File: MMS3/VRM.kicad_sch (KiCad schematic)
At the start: 32 parts, among them U3 TPS54560BDDA

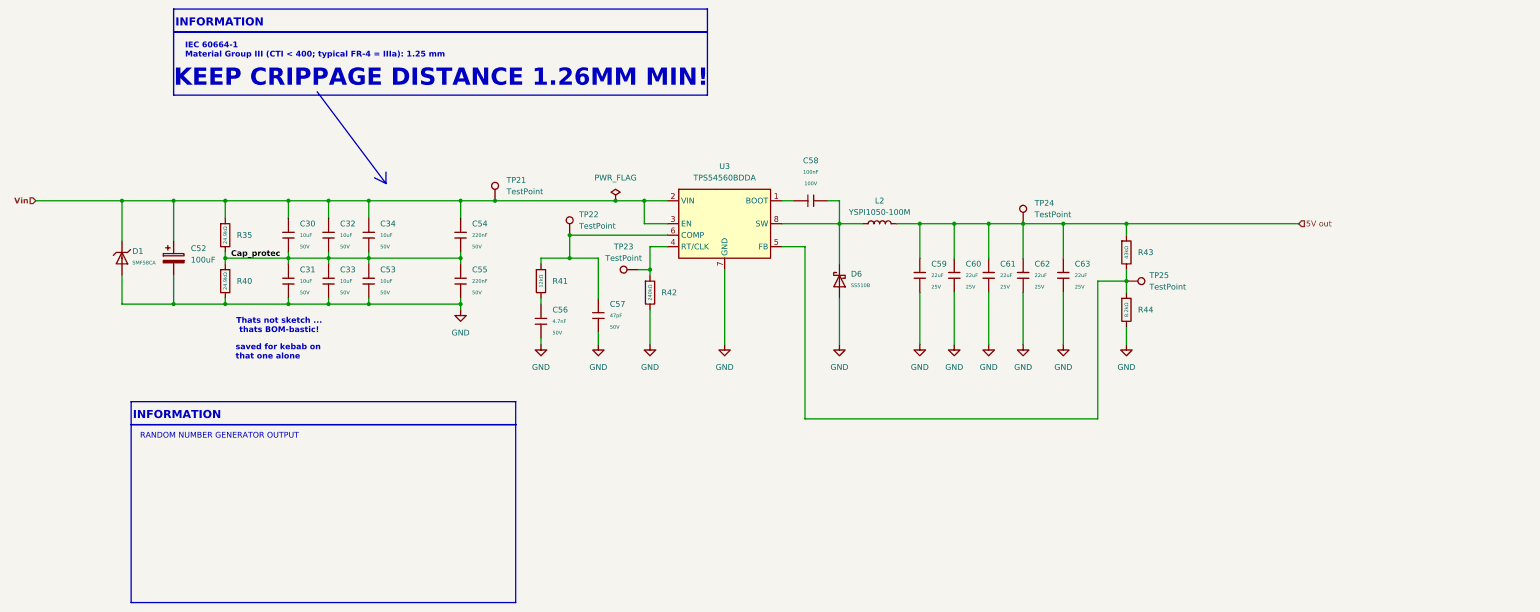
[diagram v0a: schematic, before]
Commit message: initial PCB update
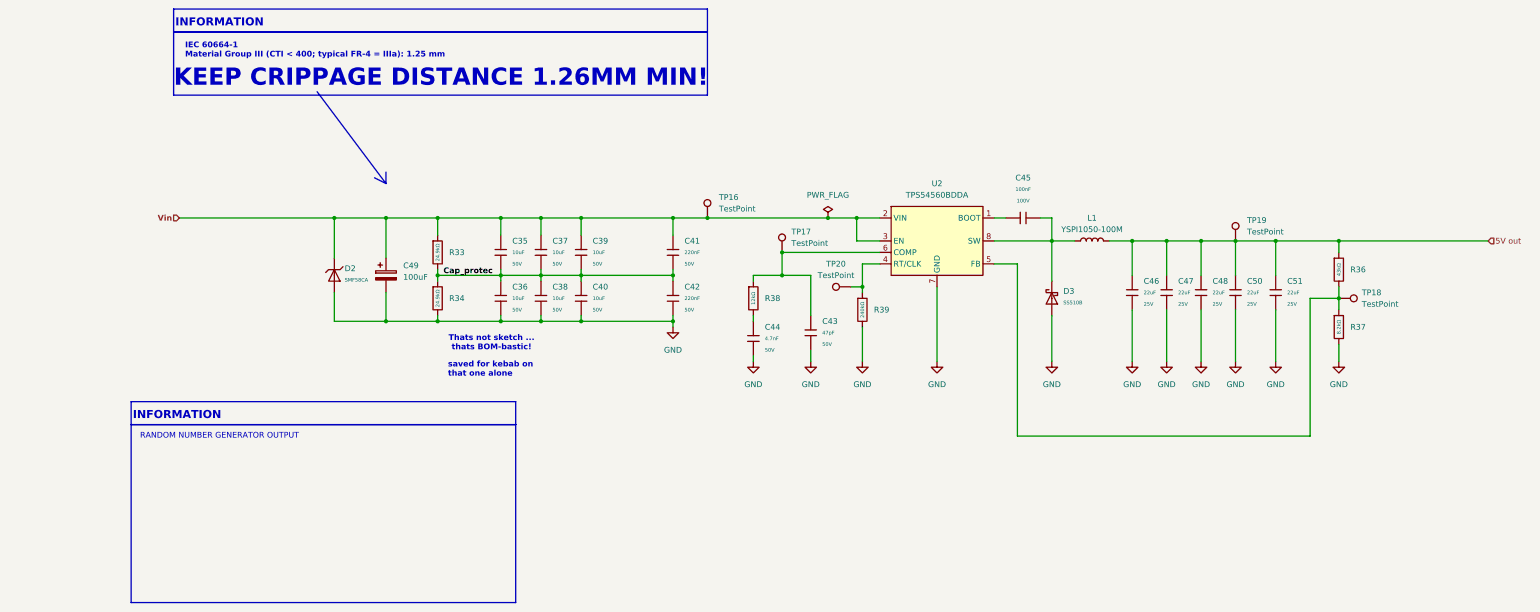
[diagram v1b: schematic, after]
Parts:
- removed C30, C31, C32, C33, C34, C53: 10uF, PCM_JLCPCB:C_0805, symbol PCM_JLCPCB-Capacitors:0805,10uF,(2)
- removed C52: 100uF, Capacitor_SMD:CP_Elec_10x10, symbol Device:C_Polarized
- removed C54, C55: 220nF, PCM_JLCPCB:C_0805, symbol PCM_JLCPCB-Capacitors:0805,220nF
- removed C56: 4.7nF, PCM_JLCPCB:C_0402, symbol PCM_JLCPCB-Capacitors:0402,4.7nF
- removed C57: 47pF, PCM_JLCPCB:C_0402, symbol PCM_JLCPCB-Capacitors:0402,47pF
- removed C58: 100nF, PCM_JLCPCB:C_0805, symbol PCM_JLCPCB-Capacitors:0805,100nF
- removed C59, C60, C61, C62, C63: 22uF, PCM_JLCPCB:C_0805, symbol PCM_JLCPCB-Capacitors:0805,22uF
- removed D1: SMF58CA, PCM_JLCPCB:D_SOD-123FL, symbol PCM_JLCPCB-Diodes:TVS-Uni,SMF58CA
- removed D6: SS510B, PCM_JLCPCB:D_SMB, symbol PCM_JLCPCB-Diodes:Schottky,SS510B
- removed L2: YSPI1050-100M, Inductor_SMD:L_Sunlord_MWSA1005S, symbol Device:L
- removed R35, R40: 24.9kΩ, PCM_JLCPCB:R_0402, symbol PCM_JLCPCB-Resistors:0402,24kΩ
- removed R41: 12kΩ, PCM_JLCPCB:R_0402, symbol PCM_JLCPCB-Resistors:0402,12kΩ
- removed R42: 240kΩ, PCM_JLCPCB:R_0603, symbol PCM_JLCPCB-Resistors:0603,240kΩ
- removed R43: 43kΩ, PCM_JLCPCB:R_0603, symbol PCM_JLCPCB-Resistors:0603,43kΩ
- removed R44: 8.2kΩ, PCM_JLCPCB:R_0402, symbol PCM_JLCPCB-Resistors:0402,8.2kΩ
- removed TP21, TP22, TP23, TP24, TP25: TestPoint, TestPoint:TestPoint_Pad_D1.0mm, symbol Connector:TestPoint
- removed U3: TPS54560BDDA, Package_SO:Texas_R-PDSO-G8_EP2.95x4.9mm_Mask2.4x3.1mm_ThermalVias, symbol Regulator_Switching:TPS54560BDDA
- added C35, C36, C37, C38, C39, C40: 10uF, PCM_JLCPCB:C_0805, symbol PCM_JLCPCB-Capacitors:0805,10uF,(2)
- added C41, C42: 220nF, PCM_JLCPCB:C_0805, symbol PCM_JLCPCB-Capacitors:0805,220nF
- added C43: 47pF, PCM_JLCPCB:C_0402, symbol PCM_JLCPCB-Capacitors:0402,47pF
- added C44: 4.7nF, PCM_JLCPCB:C_0402, symbol PCM_JLCPCB-Capacitors:0402,4.7nF
- added C45: 100nF, PCM_JLCPCB:C_0805, symbol PCM_JLCPCB-Capacitors:0805,100nF
- added C46, C47, C48, C50, C51: 22uF, PCM_JLCPCB:C_0805, symbol PCM_JLCPCB-Capacitors:0805,22uF
- added C49: 100uF, Capacitor_SMD:CP_Elec_10x10, symbol Device:C_Polarized
- added D2: SMF58CA, PCM_JLCPCB:D_SOD-123FL, symbol PCM_JLCPCB-Diodes:TVS-Uni,SMF58CA
- added D3: SS510B, PCM_JLCPCB:D_SMB, symbol PCM_JLCPCB-Diodes:Schottky,SS510B
- added L1: YSPI1050-100M, Inductor_SMD:L_Sunlord_MWSA1005S, symbol Device:L
- added R33, R34: 24.9kΩ, PCM_JLCPCB:R_0402, symbol PCM_JLCPCB-Resistors:0402,24kΩ
- added R36: 43kΩ, PCM_JLCPCB:R_0603, symbol PCM_JLCPCB-Resistors:0603,43kΩ
- added R37: 8.2kΩ, PCM_JLCPCB:R_0402, symbol PCM_JLCPCB-Resistors:0402,8.2kΩ
- added R38: 12kΩ, PCM_JLCPCB:R_0402, symbol PCM_JLCPCB-Resistors:0402,12kΩ
- added R39: 240kΩ, PCM_JLCPCB:R_0603, symbol PCM_JLCPCB-Resistors:0603,240kΩ
- added TP16, TP17, TP18, TP19, TP20: TestPoint, TestPoint:TestPoint_Pad_D1.0mm, symbol Connector:TestPoint
- added U2: TPS54560BDDA, Package_SO:Texas_R-PDSO-G8_EP2.95x4.9mm_Mask2.4x3.1mm_ThermalVias, symbol Regulator_Switching:TPS54560BDDA
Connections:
- net 5V out: now also C46.1, C47.1, C48.1, C50.1, C51.1, L1.2, R36.1, TP19.1
- net Cap_protec: now also C35.2, C36.1, C37.2, C38.1, C39.2, C40.1, C41.2, C42.1, R33.2, R34.1
- net GND: now also C36.2, C38.2, C40.2, C42.2, C43.2, C44.2, C46.2, C47.2, C48.2, C49.2, C50.2, C51.2, D2.2, D3.2, R34.2, R37.2, R39.2, U2.7 (GND), U2.9 (GND)
- net Vin: now also C35.1, C37.1, C39.1, C41.1, C49.1, D2.1, R33.1, TP16.1, U2.2 (VIN), U2.3 (EN)
- new net: C45.1, D3.1, L1.1, U2.8 (SW)
- new net: C45.2, U2.1 (BOOT)
- new net: C44.1, R38.2
- new net: C43.1, R38.1, TP17.1, U2.6 (COMP)
- new net: R39.1, TP20.1, U2.4 (RT/CLK)
- new net: R36.2, R37.1, TP18.1, U2.5 (FB)
